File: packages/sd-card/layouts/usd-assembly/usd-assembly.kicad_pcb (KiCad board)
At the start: 2 copper layers, 5 parts

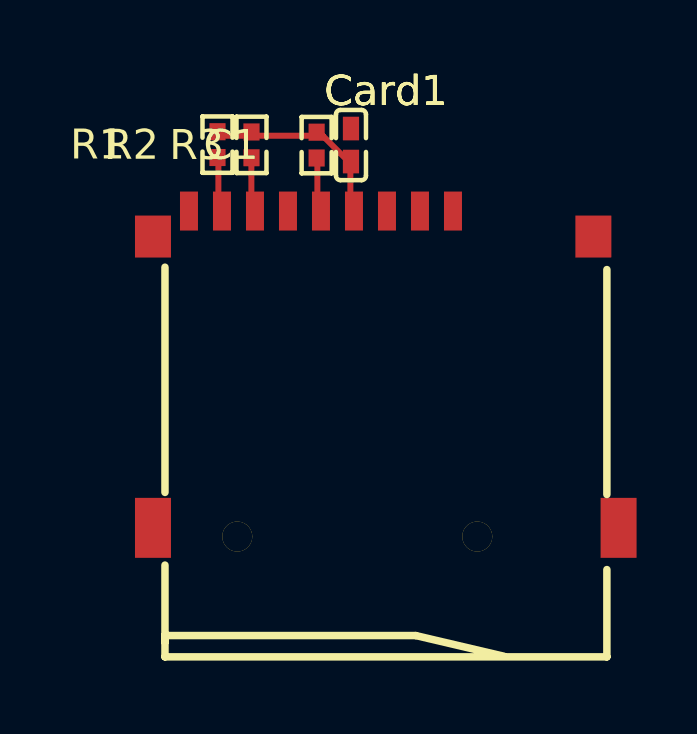
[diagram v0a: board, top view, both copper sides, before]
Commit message: bigg
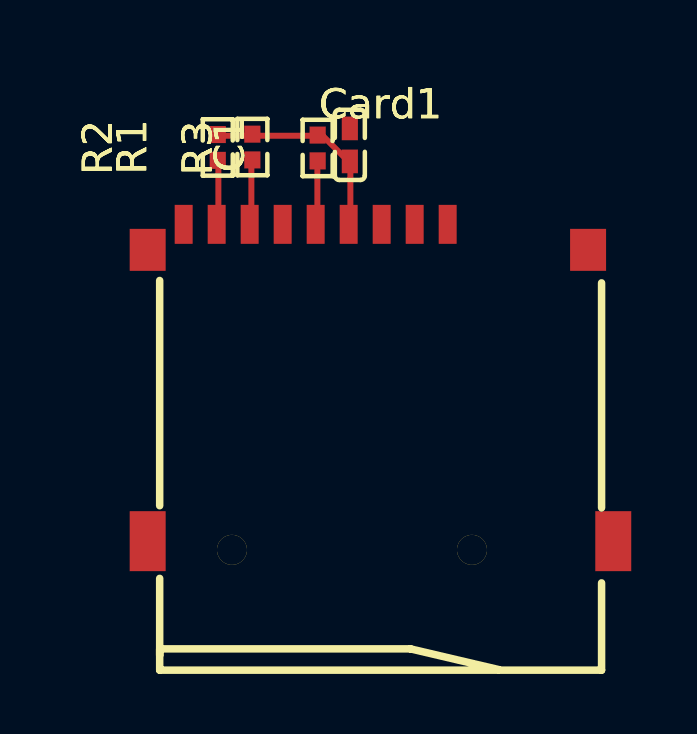
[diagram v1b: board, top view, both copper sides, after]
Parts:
- moved R1 1.16 mm to (66.6, 53.0)
- moved R2 1.13 mm to (65.4, 53.0)
- moved Card1 0.48 mm to (70.8, 60.8)
- moved R3 0.10 mm to (68.7, 53.0)
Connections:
- net DAT2 renamed pins[8]
- net line-0 renamed pins[0]
- net line-1 renamed pins[6]
- net line-2 renamed pins[7]
